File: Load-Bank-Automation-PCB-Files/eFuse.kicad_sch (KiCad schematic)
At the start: 11 parts, among them U1 TPS259470ARPWR

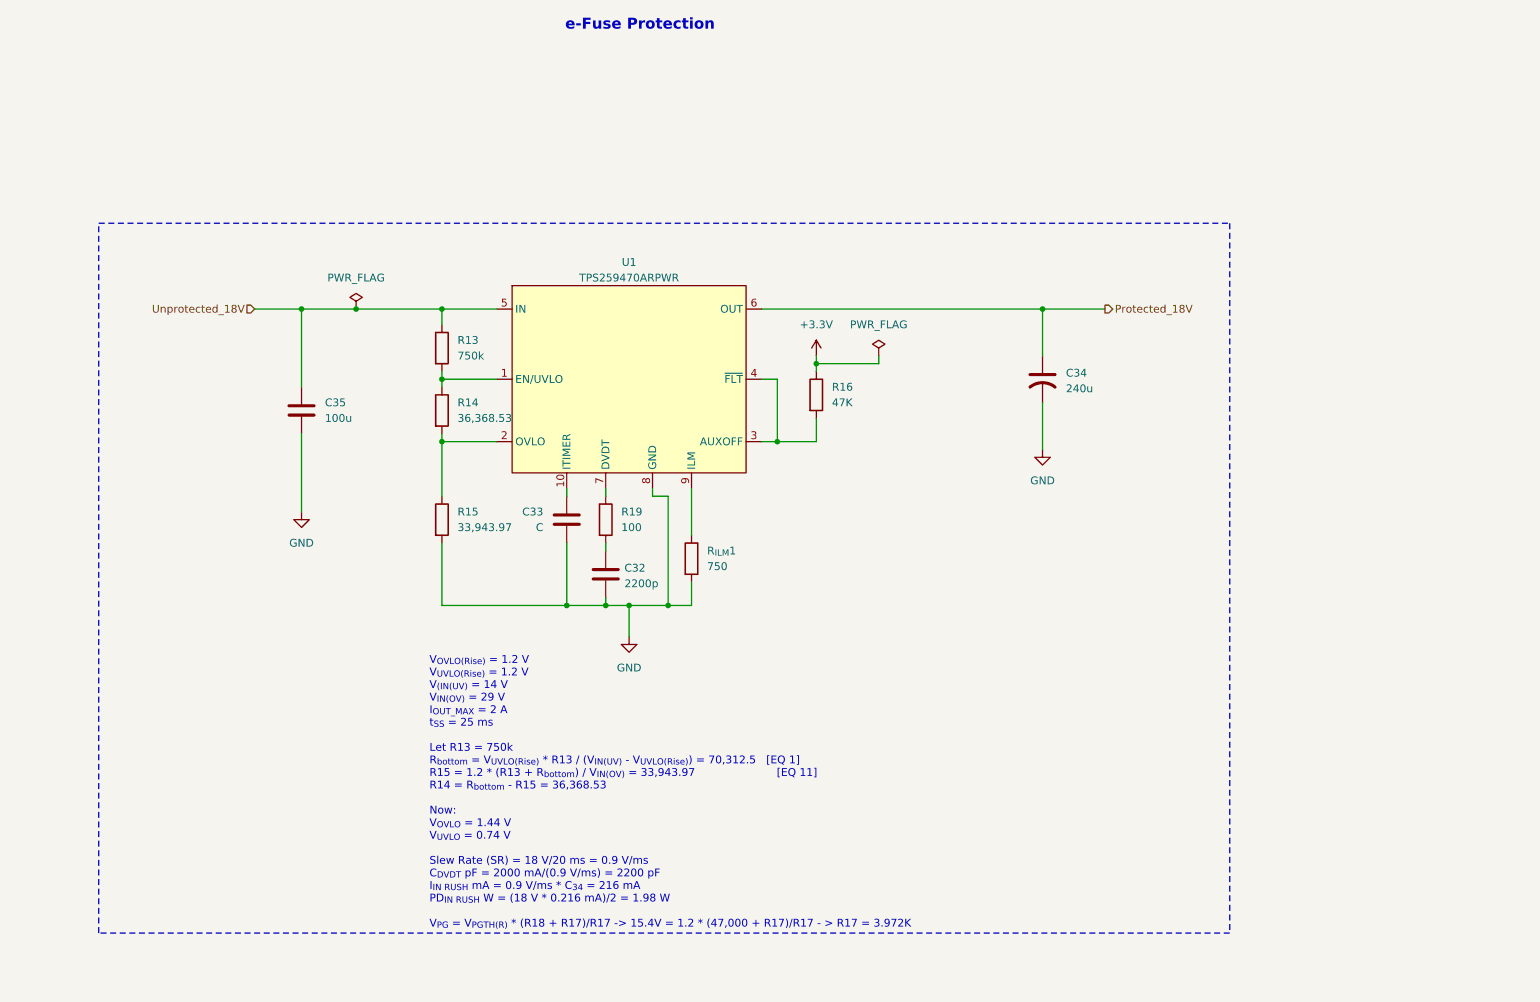
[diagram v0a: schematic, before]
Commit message: Schematic for revision
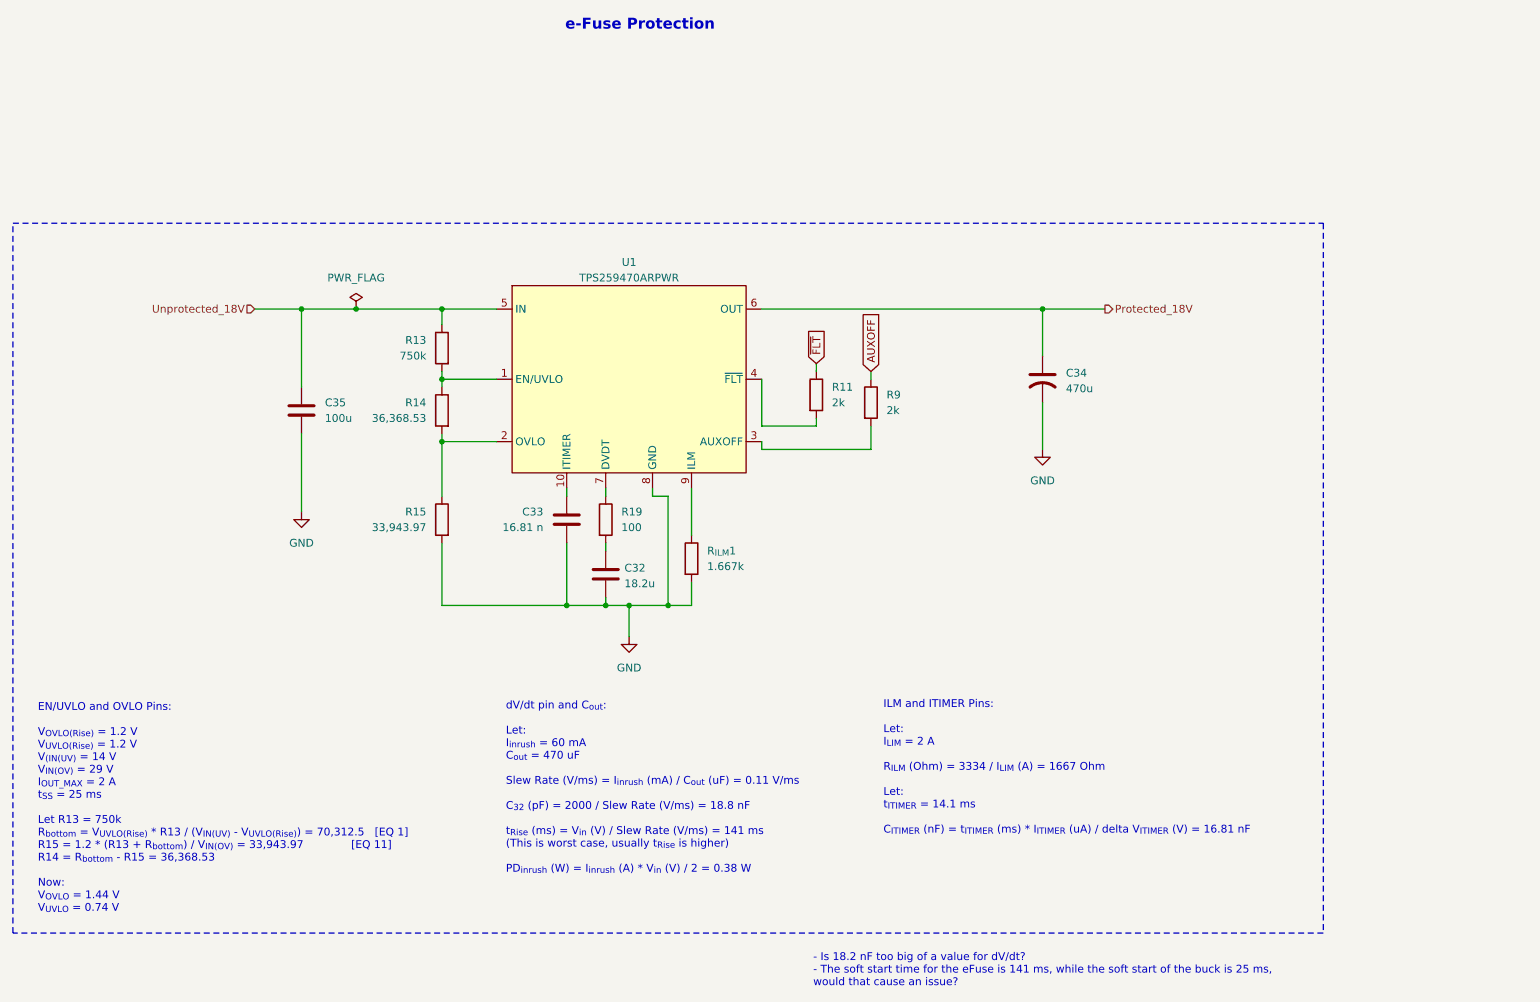
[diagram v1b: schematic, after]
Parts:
- removed R16: 47K, Resistor_SMD:R_0402_1005Metric_Pad0.72x0.64mm_HandSolder, symbol Device:R
- added R11, R9: 2k, Resistor_SMD:R_0402_1005Metric_Pad0.72x0.64mm_HandSolder, symbol Device:R
- C32: value 2200p -> 18.2u
- C33: value C -> 16.81 n
- C34: value 240u -> 470u
- R_{ILM}1: value 750 -> 1.667k
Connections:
- net at U1.4 (~{FLT}): now also R11.2; no longer U1.3 (AUXOFF)
- new net: R9.2, U1.3 (AUXOFF)
- new net AUXOFF: R9.1
- new net ~{FLT}: R11.1
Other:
- note added: "- Is 18.2 nF too big of a value for dV/dt? - The soft start time for the eFuse is 141 ms, while the soft start of the buck is 25 ms, would that cause an issue?"
- note added: "EN/UVLO and OVLO Pins: V_{OVLO(Rise)} = 1.2 V V_{UVLO(Rise)} = 1.2 V V_{(IN(UV)} = 14 V V_{IN(OV)} = 29 V I_{OUT_MAX} = 2 A t_{SS} = 25 ms Let R13 = 750k R_{bottom} = V_{UVLO(Rise)} * R13 / (V_{IN(UV)} - V_{UVLO(Rise)}) = 70,312.5 [EQ 1] R15 = 1.2 * (R13 + R_{bottom}) / V_{IN(OV)} = 33,943.97 [EQ 11] R14 = R_{bottom} - R15 = 36,368.53 Now: V_{OVLO} = 1.44 V V_{UVLO} = 0.74 V"
- note added: "ILM and ITIMER Pins: Let: I_{LIM} = 2 A R_{ILM} (Ohm) = 3334 / I_{LIM} (A) = 1667 Ohm Let: t_{ITIMER} = 14.1 ms C_{ITIMER} (nF) = t_{ITIMER} (ms) * I_{ITIMER} (uA) / delta V_{ITIMER} (V) = 16.81 nF"
- note added: "dV/dt pin and C_{out}: Let: I_{inrush} = 60 mA C_{out} = 470 uF Slew Rate (V/ms) = I_{inrush} (mA) / C_{out} (uF) = 0.11 V/ms C_{32} (pF) = 2000 / Slew Rate (V/ms) = 18.8 nF t_{Rise} (ms) = V_{in} (V) / Slew Rate (V/ms) = 141 ms (This is worst case, usually t_{Rise} is higher) PD_{inrush} (W) = I_{inrush} (A) * V_{in} (V) / 2 = 0.38 W"
- note removed: "V_{OVLO(Rise)} = 1.2 V V_{UVLO(Rise)} = 1.2 V V_{(IN(UV)} = 14 V V_{IN(OV)} = 29 V I_{OUT_MAX} = 2 A t_{SS} = 25 ms Let R13 = 750k R_{bottom} = V_{UVLO(Rise)} * R13 / (V_{IN(UV)} - V_{UVLO(Rise)}) = 70,312.5 [EQ 1] R15 = 1.2 * (R13 + R_{bottom}) / V_{IN(OV)} = 33,943.97 [EQ 11] R14 = R_{bottom} - R15 = 36,368.53 Now: V_{OVLO} = 1.44 V V_{UVLO} = 0.74 V Slew Rate (SR) = 18 V/20 ms = 0.9 V/ms C_{DV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"
